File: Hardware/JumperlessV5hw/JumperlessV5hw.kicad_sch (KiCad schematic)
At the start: 183 parts, among them J1 Debug, J11 TopOutMAIN, J12 TopInMAIN, J13 BottomInMAIN, J14 5V, J15 BottomOutMAIN, J1711 Conn_01x15, J1712 Conn_01x15, J2 USB_C_Receptacle_USB2.0_16P, J3 ProbeJack, J4 Breadboard, J5 ProbeHeader, J6 CH446Q, J7 DaisyChain_OUT, J8 DaisyChain_IN, K1 CH446Q, SW1 BOOT, SW3 RotaryEncoder_Switch, U1 LT1054, U10 L272D, U11 LM324, U1806 MCP4728, U1807 L272D, U1808 MCP23S17_ML, U2 NCP1117-3.3_SOT223, U3 INA219, U4 INA219, U7 LM324, U8 W25Q128JVS, U9 RP2040, Y1 ABLS-12.000MHZ-B4-T

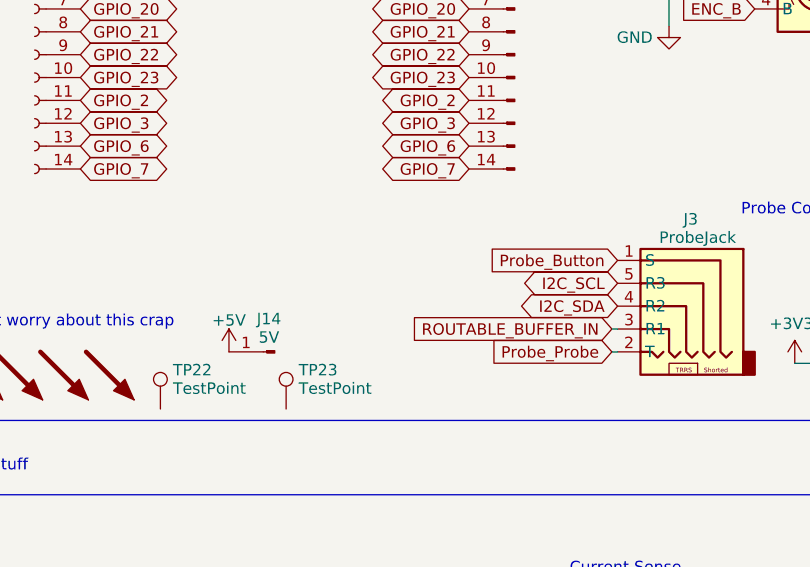
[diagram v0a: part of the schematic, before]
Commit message: Getting probing to work and a bunch of other stuff
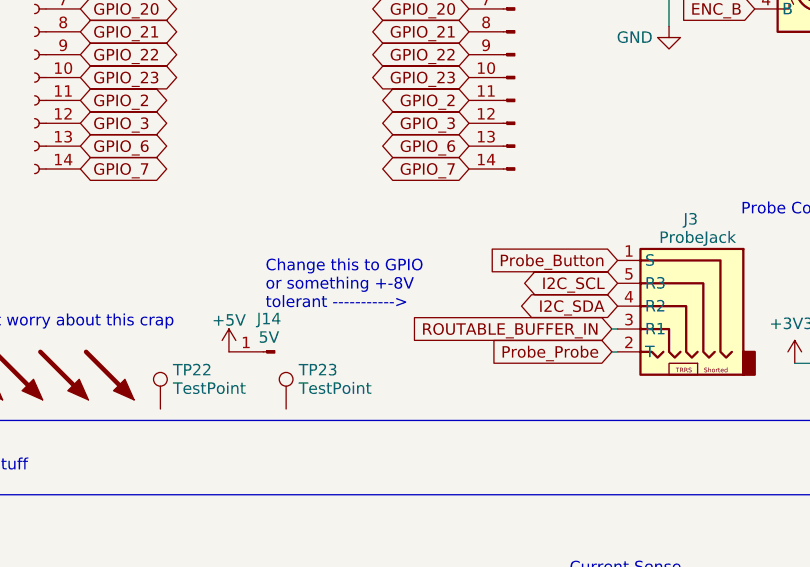
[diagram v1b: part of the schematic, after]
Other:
- note added: "Change this to GPIO or something +-8V tolerant ----------->"
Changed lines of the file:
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@@
+		)
+	)
+	(text "Change this to GPIO\nor something +-8V \ntolerant ----------->"
+		(exclude_from_sim no)
+		(at 653.034 128.524 0)
+		(effects
+			(font
+				(size 1.27 1.27)
+			)
+			(justify left)
 		)
 	)
